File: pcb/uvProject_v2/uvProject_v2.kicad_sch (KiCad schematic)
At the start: 22 parts, among them J1 RTC Module, J2 RESET, J3 UART, J4 BOOT, J5 POWER, J6 UV sensor, J7 Micro SD, U1 LM1117-3.3, U2 ESP8266-12E/ESP-12E

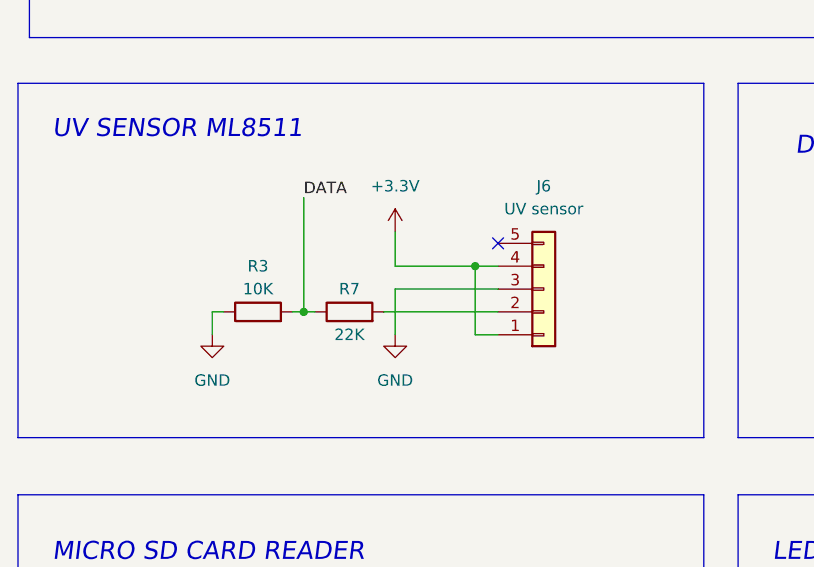
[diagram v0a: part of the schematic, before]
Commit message: update:pcb
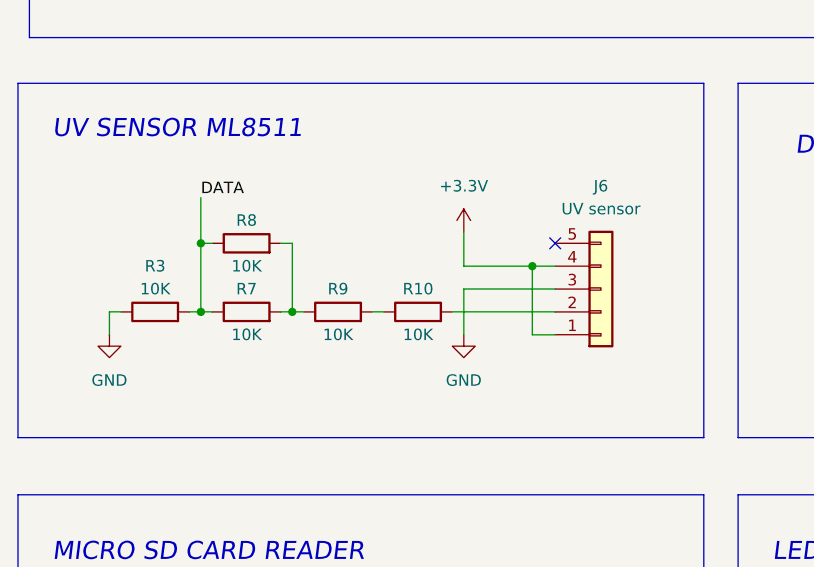
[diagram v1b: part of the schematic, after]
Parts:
- added R7, R8, R9: 10K, Resistor_SMD:R_1206_3216Metric_Pad1.30x1.75mm_HandSolder, symbol Device:R
- R10: renamed from R7; value 22K -> 10K
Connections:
- net DATA: now also R7.1, R8.1; no longer R10.1
- new net: R7.2, R8.2, R9.1
- new net: R10.1, R9.2
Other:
- moved on the sheet: J6, R10, R3
